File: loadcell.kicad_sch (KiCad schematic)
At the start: 6 parts, among them IC3 NAU7802SGI, J3 691412120004B

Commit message: changes
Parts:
- IC3: footprint SOIC127P600X175-16N -> Library:SOIC127P600X175-16N
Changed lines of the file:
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@@
 			)
 		)
-		(property "Footprint" "SOIC127P600X175-16N"
+		(property "Footprint" "Library:SOIC127P600X175-16N"
 			(at 148.59 155.88 0)
 			(effects

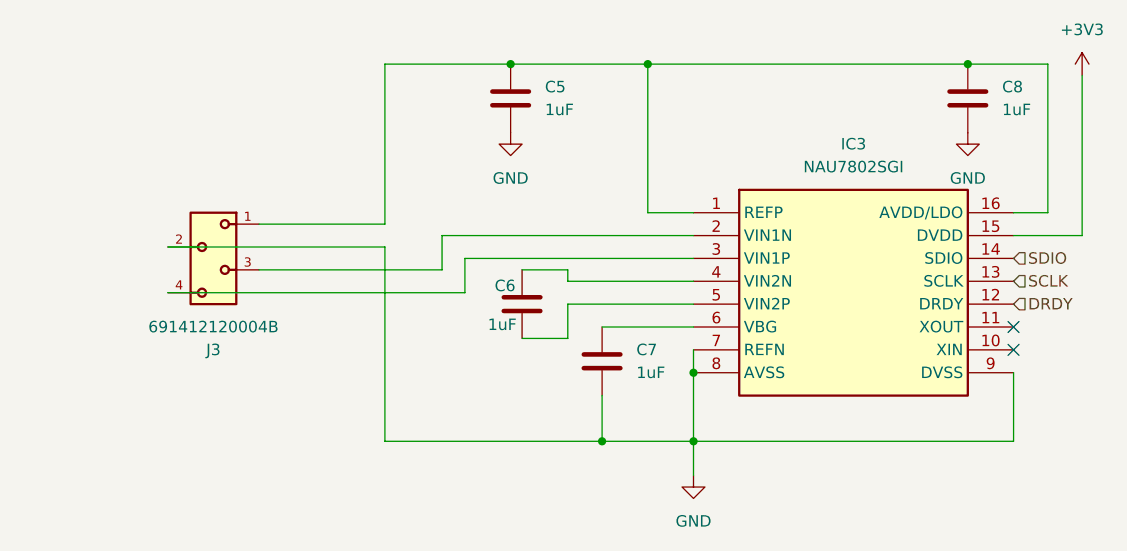
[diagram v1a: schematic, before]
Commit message: lots of change
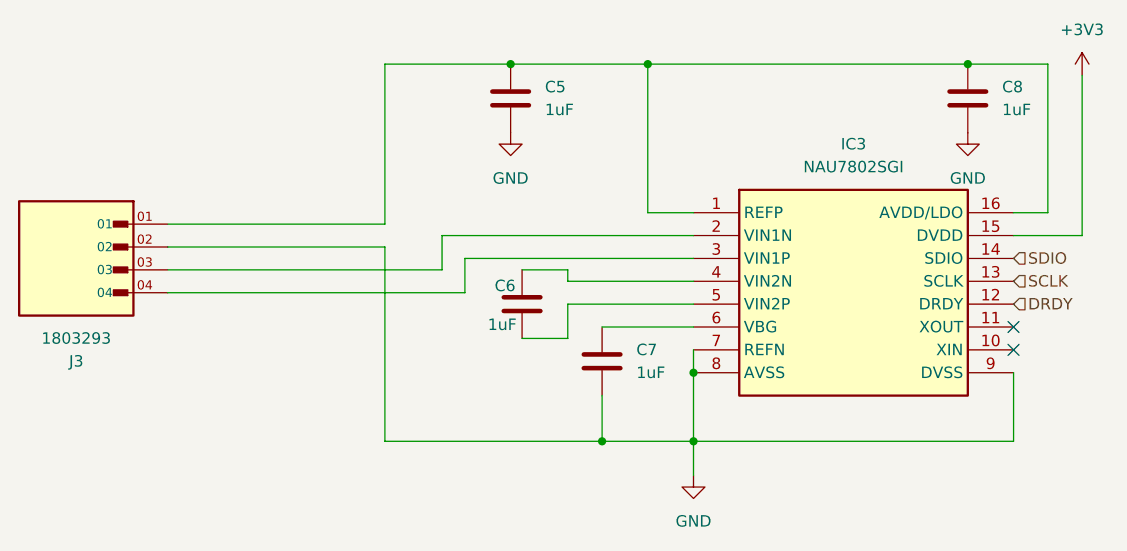
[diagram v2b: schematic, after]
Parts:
- removed J3: 691412120004B, Library:691412120004B, symbol 691412120004B:691412120004B
- added J3: 1803293, Library:PHOENIX_1803293, symbol afterburner_symbolic:1803293
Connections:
- net GND: now also J3.02
- net at C5.1, C8.1, IC3.1 (REFP)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: now also J3.01
- net at IC3.2 (VIN1N): now also J3.03
- net at IC3.3 (VIN1P): now also J3.04
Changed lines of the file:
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@@
+	(wire
+		(pts
+			(xy 58.42 62.23) (xy 82.55 62.23)
+		)
+		(stroke
+			(width 0)
+			(type default)
+		)
+	)
 	(wire
 		(pts
@@
 	(wire
 		(pts
-			(xy 68.58 62.23) (xy 82.55 62.23)
-		)
-		(stroke
-			(width 0)
-			(type default)
-		)
-	)
-	(wire
-		(pts
 			(xy 111.76 44.45) (xy 147.32 44.45)
 		)
@@
 	(wire
 		(pts
-			(xy 68.58 67.31) (xy 88.9 67.31)
-		)
-		(stroke
-			(width 0)
-			(type default)
-		)
-	)
-	(wire
-		(pts
 			(xy 116.84 86.36) (xy 116.84 90.17)
 		)
@@
 		(pts
 			(xy 91.44 69.85) (xy 91.44 66.04)
+		)
+		(stroke
+			(width 0)
+			(type default)
+		)
+	)
+	(wire
+		(pts
+			(xy 58.42 67.31) (xy 88.9 67.31)
 		)
 		(stroke
@@
 	)
 	(symbol
+		(lib_id "afterburner_symbolic:1803293")
+		(at 48.26 67.31 0)
+		(mirror y)
+		(unit 1)
+		(exclude_from_sim no)
+		(in_bom yes)
+		(on_board yes)
+		(dnp no)
+		(property "Reference" "J3"
+			(at 48.26 77.47 0)
+			(effects
+				(font
+					(size 1.27 1.27)
+				)
+			)
+		)
+		(property "Value" "1803293"
+			(at 48.26 74.93 0)
+			(effects
+				(font
+					(size 1.27 1.27)
+				)
+			)
+		)
+		(property "Footprint" "Library:PHOENIX_1803293"
+			(at 48.26 67.31 0)
+			(effects
+				(font
+					(size 1.27 1.27)
+				)
+				(justify bottom)
+				(hide yes)
+			)
+		)
+		(property "Datasheet" ""
+			(at 48.26 67.31 0)
+			(effects
+				(font
+					(size 1.27 1.27)
+				)
+				(hide yes)
+			)
+		)
+		(property "Description" ""
+			(at 48.26 67.31 0)
+			(effects
+				(font
+					(size 1.27 1.27)
+				)
+				(hide yes)
+			)
+		)
+		(property "PARTREV" "08.06.2015"
+			(at 48.26 67.31 0)
+			(effects
+				(font
+					(size 1.27 1.27)
+				)
+				(justify bottom)
+				(hide yes)
+			)
+		)
+		(property "STANDARD" "Manufacturer Recommendations"
+			(at 48.26 67.31 0)
+			(effects
+				(font
+					(size 1.27 1.27)
+				)
+				(justify bottom)
+				(hide yes)
+			)
+		)
+		(property "MANUFACTURER" "Phoenix Contact"
+			(at 48.26 67.31 0)
+			(effects
+				(font
+					(size 1.27 1.27)
+				)
+				(justify bottom)
+				(hide yes)
+			)
+		)
+		(pin "03"
+		)
+		(pin "04"
+		)
+		(pin "02"
+		)
+		(pin "01"
+		)
+		(instances
+			(project "afterburner"
+				(path "/2e03126f-90c3-49c2-bb02-7889a4a780ce/d4aa8317-4dd0-460d-8e3e-edb5da807fd1"
+					(reference "J3")
+					(unit 1)
+				)
+			)
+		)
+	)
+	(symbol
 		(lib_id "Device:C")
 		(at 106.68 77.47 0)
@@
 					(unit 1)
 				)
-			)
-		)
-	)
-	(symbol
-		(lib_id "691412120004B:691412120004B")
-		(at 63.5 64.77 90)
-		(mirror x)
-		(unit 1)
-		(exclude_from_sim no)
-		(in_bom yes)
-		(on_board yes)
-		(dnp no)
-		(property "Reference" "J3"
-			(at 63.5 76.2 90)
-			(effects
-				(font
-					(size 1.27 1.27)
-				)
-			)
-		)
-		(property "Value" "691412120004B"
-			(at 63.5 73.66 90)
-			(effects
-				(font
-					(size 1.27 1.27)
-				)
-			)
-		)
-		(property "Footprint" "Library:691412120004B"
-			(at 63.5 64.77 0)
-			(effects
-				(font
-					(size 1.27 1.27)
-				)
-				(justify bottom)
-				(hide yes)
-			)
-		)
-		(property "Datasheet" ""
-			(at 63.5 64.77 0)
-			(effects
-				(font
-					(size 1.27 1.27)
-				)
-				(hide yes)
-			)
-		)
-		(property "Description" ""
-			(at 63.5 64.77 0)
-			(effects
-				(font
-					(size 1.27 1.27)
-				)
-				(hide yes)
-			)
-		)
-		(pin "2"
-		)
-		(pin "3"
-		)
-		(pin "1"
-		)
-		(pin "4"
-		)
-		(instances
-			(project "first_project"
-				(path "/2e03126f-90c3-49c2-bb02-7889a4a780ce/d4aa8317-4dd0-460d-8e3e-edb5da807fd1"
-					(reference "J3")
-					(unit 1)
-				)
